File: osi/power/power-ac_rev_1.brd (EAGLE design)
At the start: 25.4 x 25.4 mm, 8 parts, among them IC1 TINY24/44/84-PU

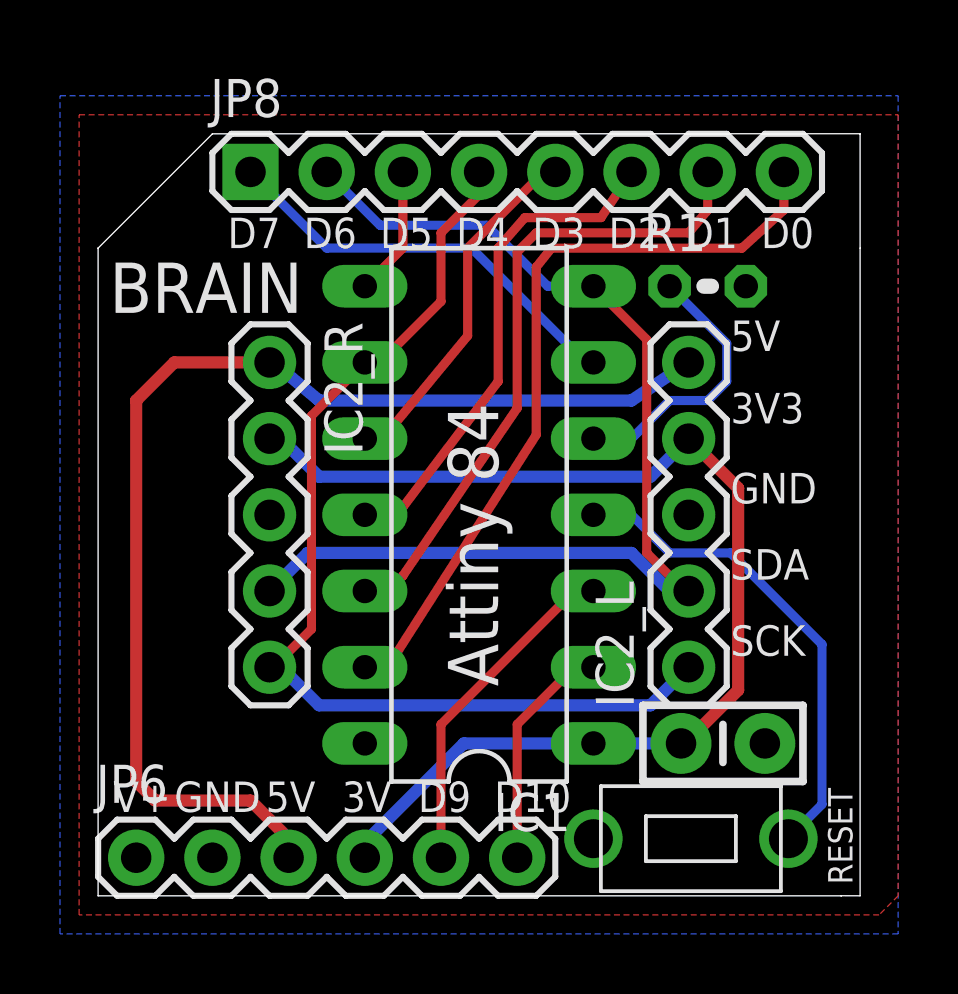
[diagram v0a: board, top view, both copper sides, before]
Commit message: control brain
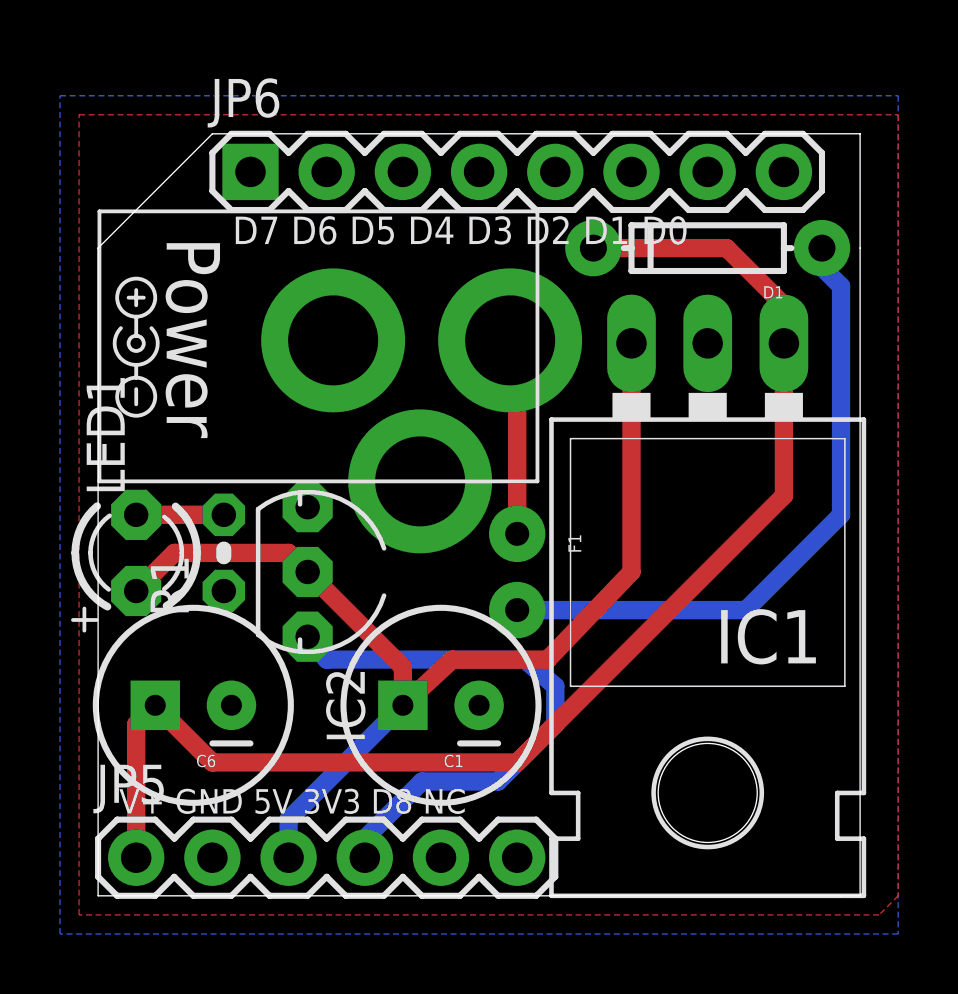
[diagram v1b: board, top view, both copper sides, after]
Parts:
- removed IC2_L, IC2_R: (no value), SparkFun_mod:1X05
- removed JP8: (no value), SparkFun:1X08
- added C6: (no value), SparkFun:CPOL-RADIAL-100UF-25V
- added D1: (no value), SparkFun:DIODE-1N4148
- added F1: PTCPTH, SparkFun_mod:PTC
- added IC2: (no value), adafruit:TO92-INLINE
- added JP5: (no value), SparkFun:1X06
- added LED1: (no value), adafruit:LED3MM
- added U$2: (no value), DC_SYM:DC_POS_CTR
- added U$3: (no value), DC_SYM:DC_POS_CTR-BOTTOM
- C1: device SparkFun:CAP-PTH-SMALL-KIT -> SparkFun:CPOL-RADIAL-100UF-25V
- IC1: value TINY24/44/84-PU -> (none); device avr-7:DIL14 -> SparkFun:TO-220-ALT
- JP6: device SparkFun:1X06 -> SparkFun:1X08
- R1: device adafruit_mod:0204V -> adafruit:0204V
- U$1: value PTS635_SWITCH -> 2.1MMJACKTHM; device _my-parts:PTS635_SWITCH -> adafruit:PJ-102A
- moved JP6 23.2 mm to (5.08, 24.1)
- moved U$1 20.4 mm to (4.45, 18.4), turned to 90 degrees
- moved R1 18.4 mm to (4.19, 11.4), turned to 90 degrees
- moved C1 9.48 mm to (11.4, 6.35)
- moved IC1 7.85 mm to (20.3, 14.6), turned to 180 degrees
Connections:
- removed net D10: IC1.2, JP6.6
- removed net RESET: IC1.4, U$1.P$2
- new net N$1: F1.P$1, U$1.TIP
- new net N$2: LED1.K, R1.2
- new net N$3: D1.A, F1.P$2
- net +3V3: now also IC2.3, JP5.4; no longer C1.2, IC1.1, IC2_L.4, IC2_R.2, JP6.4
- net +5V: now also C1.1, IC1.OUT, IC2.2, JP5.3, LED1.A; no longer IC2_L.5, IC2_R.1, JP6.3
- net AREF_D0: now also JP6.8; no longer IC1.13, JP8.8
- net D1: now also JP6.7; no longer IC1.12, JP8.7
- net D2: now also JP6.6; no longer IC1.11, JP8.6
- net D3: now also JP6.5; no longer IC1.10, JP8.5
- net D5: now also JP6.3; no longer IC1.8, JP8.3
- net D7: now also JP6.1; no longer IC1.6, JP8.1
- net D8: now also JP5.5; no longer IC1.5, R1.1
- net D9: now also JP5.6; no longer IC1.3, JP6.5
- net GND: now also C1.2, C6.2, IC1.GND, IC2.1, JP5.2, R1.1, U$1.RING; no longer C1.1, IC1.14, IC2_L.3, IC2_R.3, JP6.2, R1.2, U$1.P$1
- net SCL_D4: now also JP6.4; no longer IC1.9, IC2_L.1, IC2_R.5, JP8.4
- net SDA_D6: now also JP6.2; no longer IC1.7, IC2_L.2, IC2_R.4, JP8.2
- net V+: now also C6.1, D1.C, IC1.IN, JP5.1; no longer JP6.1
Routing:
- net V+: track 0.00 -> 44.3 mm
- net SDA_D6: track 37.0 -> 0.00 mm
- net SCL_D4: track 34.8 -> 0.00 mm
- net AREF_D0: track 25.9 -> 0.00 mm
- net D1: track 21.7 -> 0.00 mm
- net N$3: track 0.00 -> 21.3 mm
- net +3V3: track 39.4 -> 18.8 mm
- net D2: track 16.8 -> 0.00 mm
- net RESET: track 16.3 -> 0.00 mm
- net D7: track 14.1 -> 0.00 mm
- net D3: track 11.9 -> 0.00 mm
- net D9: track 11.4 -> 0.00 mm
- net D8: track 9.20 -> 0.00 mm
- net D10: track 7.77 -> 0.00 mm
- net N$1: track 0.00 -> 6.55 mm
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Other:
- board text added: "D0 D1 D2 D3 D4 D5 D6 D7"
- board text added: "D7 D6 D5 D4 D3 D2 D1 D0"
- board text added: "NC D8 3V3 5V GND V+"
- board text added: "Power"
- board text added: "Power-AC Rev 1 Feb 12"
- board text added: "V+ GND 5V 3V3 D8 NC"
- board text removed: "3V"
- board text removed: "3V3"
- board text removed: "5V"
- board text removed: "Attiny 84"
- board text removed: "BRAIN"
- board text removed: "Brain Rev 1 Feb 12"
- board text removed: "D0"
- board text removed: "D1"
- board text removed: "D10"
- board text removed: "D2"
- board text removed: "D3"
- board text removed: "D4"
- board text removed: "D5"
- board text removed: "D6"
- board text removed: "D7"
- board text removed: "D9"
- board text removed: "GND"
- board text removed: "RESET"
- board text removed: "SCK"
- board text removed: "SDA"
- board text removed: "V+"
